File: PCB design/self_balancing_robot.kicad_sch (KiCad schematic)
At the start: 31 parts, among them J1 I2C, J2 Analog, J3 left_engine, J4 right_engine, J5 L293D_left, J6 SPI, J7 UART, J8 L293D_right, J9 input_supply, SW1 SW_Push, U1 ATmega328P-A, U4 LP2985-3.3, U5 NCP1117-5.0_SOT223, Y1 Crystal

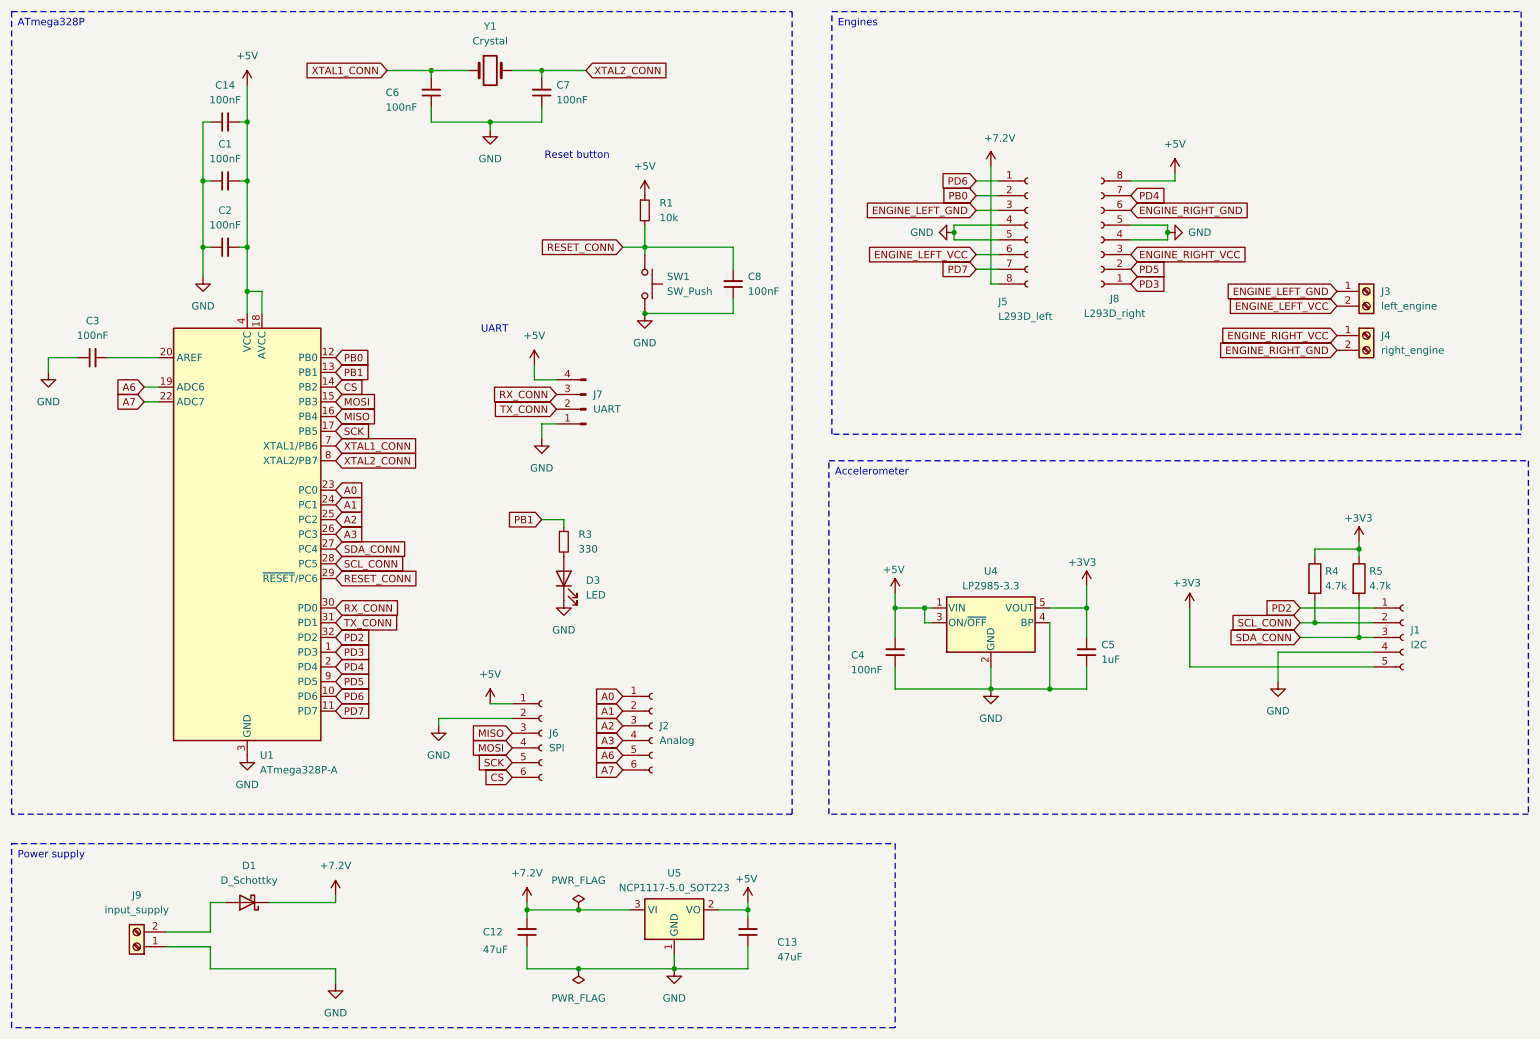
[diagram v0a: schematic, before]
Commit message: Update in PCB - almost finish version
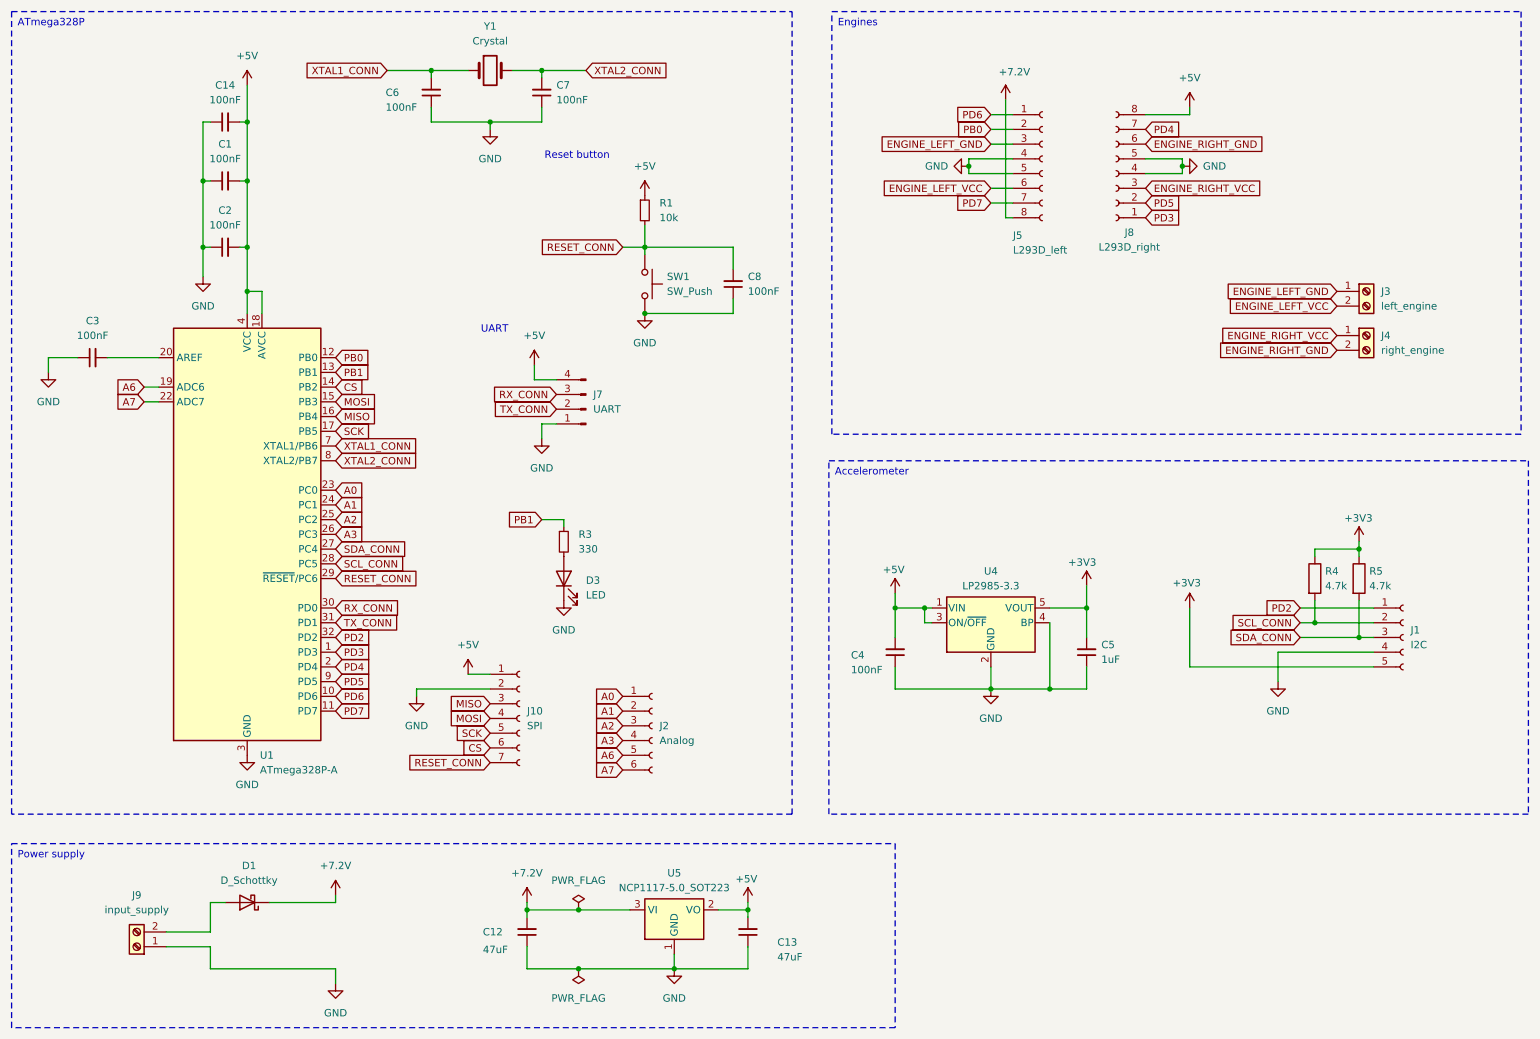
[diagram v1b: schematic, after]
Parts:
- removed J6: SPI, Connector_PinSocket_2.54mm:PinSocket_1x06_P2.54mm_Vertical, symbol Connector:Conn_01x06_Socket
- added J10: SPI, Connector_PinSocket_2.54mm:PinSocket_1x07_P2.54mm_Vertical, symbol Connector:Conn_01x07_Socket
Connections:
- net +5V: now also J10.1 (Pin_1)
- net CS: now also J10.6 (Pin_6)
- net GND: now also J10.2 (Pin_2)
- net MISO: now also J10.3 (Pin_3)
- net MOSI: now also J10.4 (Pin_4)
- net RESET_CONN: now also J10.7 (Pin_7)
- net SCK: now also J10.5 (Pin_5)
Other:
- moved on the sheet: J5, J8

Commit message: Cleaning in files part 1
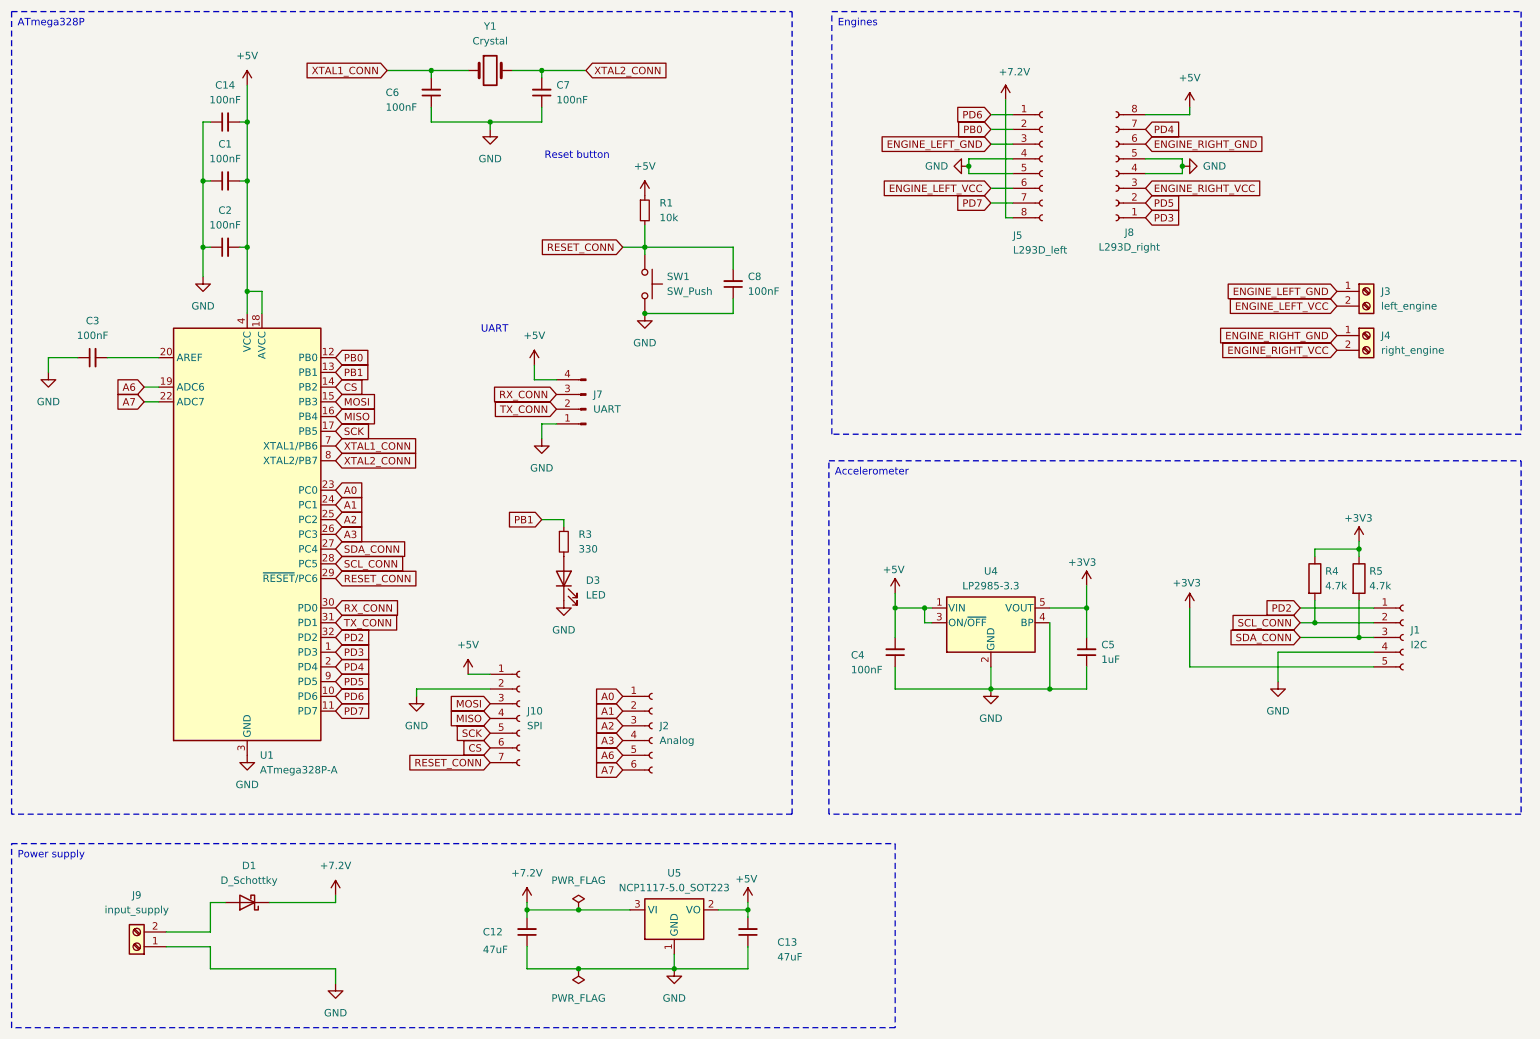
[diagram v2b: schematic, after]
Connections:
- net ENGINE_RIGHT_GND: now also J4.1 (Pin_1); no longer J4.2 (Pin_2)
- net ENGINE_RIGHT_VCC: now also J4.2 (Pin_2); no longer J4.1 (Pin_1)
- net MISO: now also J10.4 (Pin_4); no longer J10.3 (Pin_3)
- net MOSI: now also J10.3 (Pin_3); no longer J10.4 (Pin_4)
